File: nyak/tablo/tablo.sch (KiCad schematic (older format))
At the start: 109 parts

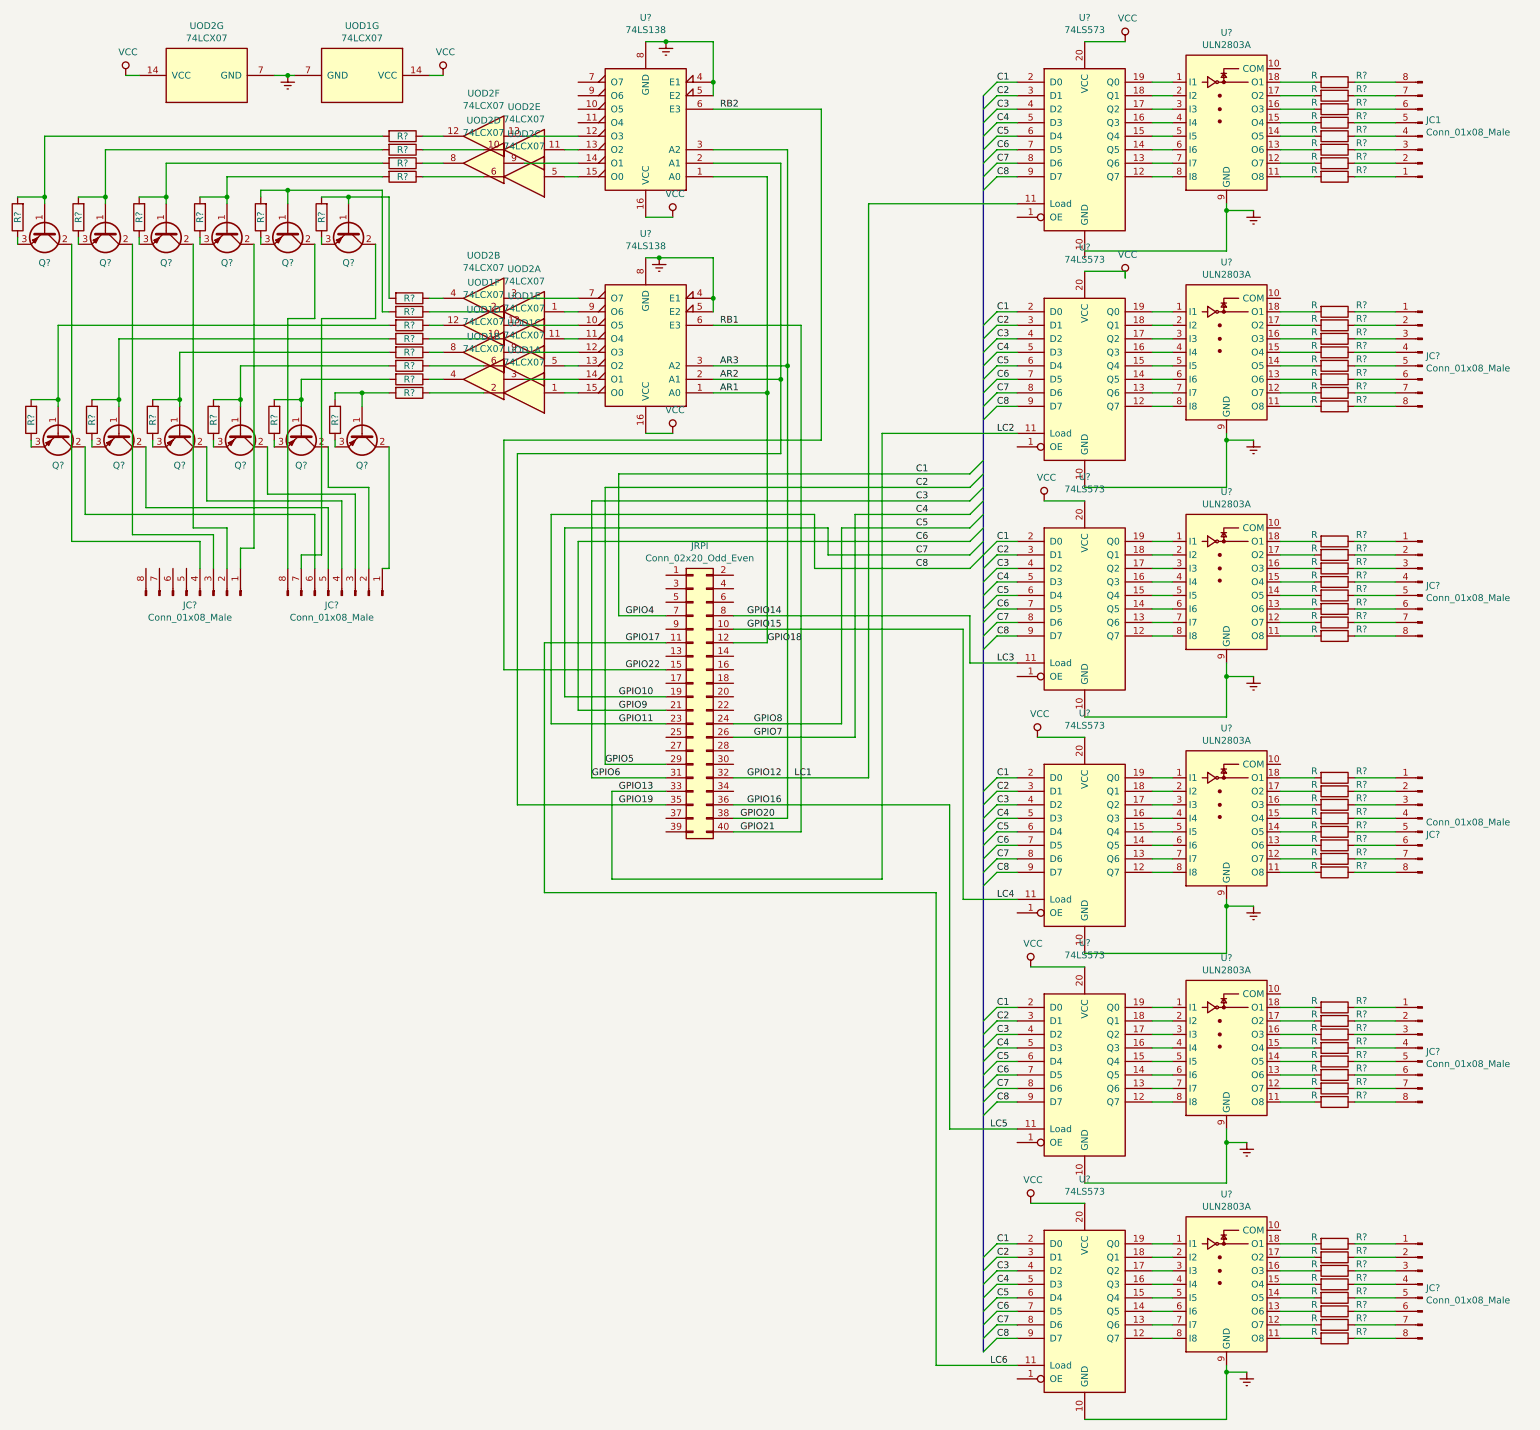
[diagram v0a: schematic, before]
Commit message: footprints added
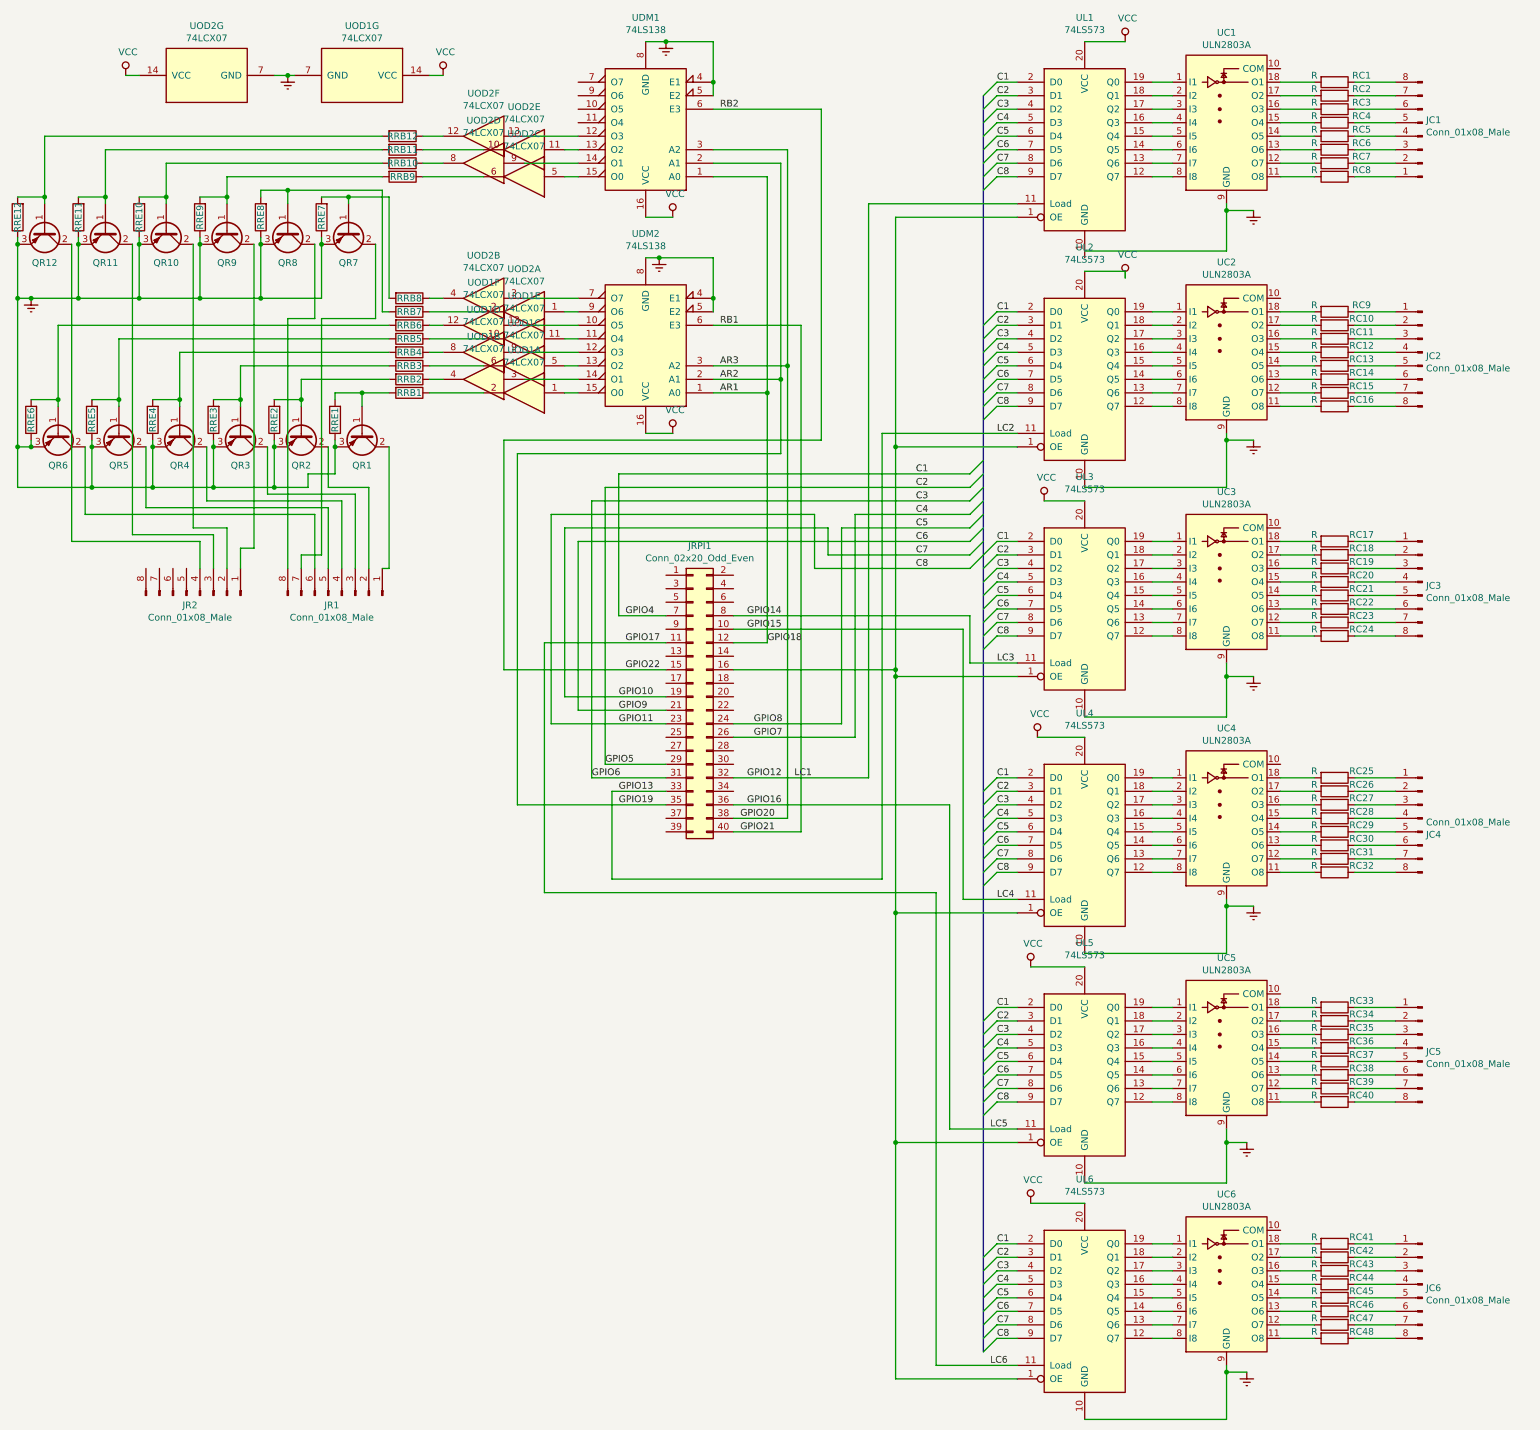
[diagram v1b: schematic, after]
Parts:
- JC1: footprint (none) -> Connector_PinHeader_2.54mm:PinHeader_1x08_P2.54mm_Vertical
- JC2, JC3, JC4, JC5, JC6, JR1, JR2: renamed from JC?; footprint (none) -> Connector_PinHeader_2.54mm:PinHeader_1x08_P2.54mm_Vertical
- JRPI1: renamed from JRPI; footprint (none) -> Connector_PinSocket_2.54mm:PinSocket_2x20_P2.54mm_Vertical
- QR1, QR10, QR11, QR12, QR2, QR3, QR4, QR5, QR6, QR7, QR8, QR9: renamed from Q?; footprint (none) -> Package_TO_SOT_THT:TO-220-3_Vertical
- RC1, RC10, RC11, RC12, RC13, RC14, RC15, RC16, RC17, RC18, RC19, RC2, RC20, RC21, RC22, RC23, RC24, RC25, RC26, RC27, RC28, RC29, RC3, RC30, RC31, RC32, RC33, RC34, RC35, RC36, RC37, RC38, RC39, RC4, RC40, RC41, RC42, RC43, RC44, RC45, RC46, RC47, RC48, RC5, RC6, RC7, RC8, RC9, RRB1, RRB10, RRB11, RRB12, RRB2, RRB3, RRB4, RRB5, RRB6, RRB7, RRB8, RRB9, RRE1, RRE10, RRE11, RRE12, RRE2, RRE3, RRE4, RRE5, RRE6, RRE7, RRE8, RRE9: renamed from R?; footprint (none) -> Resistor_THT:R_Axial_DIN0204_L3.6mm_D1.6mm_P7.62mm_Horizontal
- UC1, UC2, UC3, UC4, UC5, UC6: renamed from U?; footprint (none) -> Package_DIP:DIP-18_W7.62mm
- UDM1, UDM2: renamed from U?; footprint (none) -> Package_DIP:DIP-16_W7.62mm
- UL1, UL2, UL3, UL4, UL5, UL6: renamed from U?; footprint (none) -> Package_DIP:DIP-20_W7.62mm
- UOD1, UOD2: footprint (none) -> Package_DIP:DIP-14_W7.62mm
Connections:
- net Earth: now also QR1.3 (E), QR10.3 (E), QR11.3 (E), QR12.3 (E), QR2.3 (E), QR3.3 (E), QR4.3 (E), QR5.3 (E), QR6.3 (E), QR7.3 (E), QR8.3 (E), QR9.3 (E), RRE1.1, RRE10.1, RRE11.1, RRE12.1, RRE2.1, RRE3.1, RRE4.1, RRE5.1, RRE6.1, RRE7.1, RRE8.1, RRE9.1
- net at UL1.1 (OE): now also JRPI1.16 (Pin_16), UL2.1 (OE), UL3.1 (OE), UL4.1 (OE), UL5.1 (OE), UL6.1 (OE)

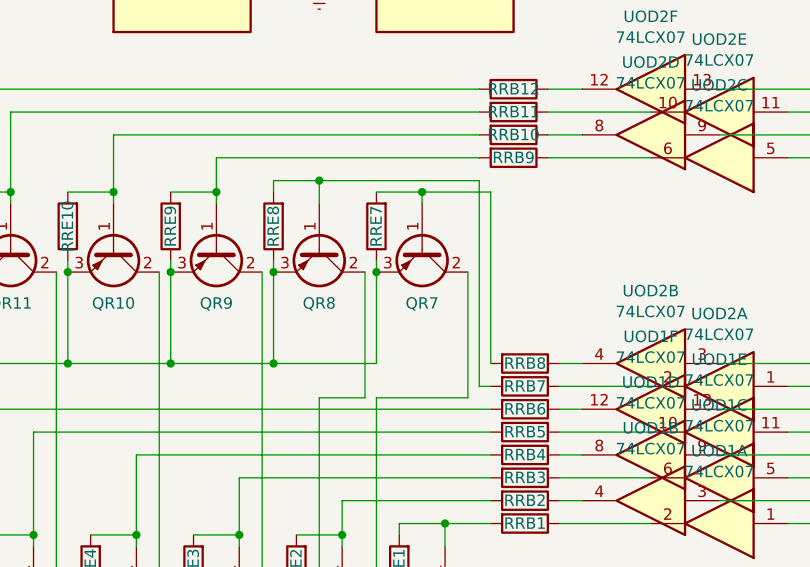
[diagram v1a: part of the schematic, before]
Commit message: more tracks
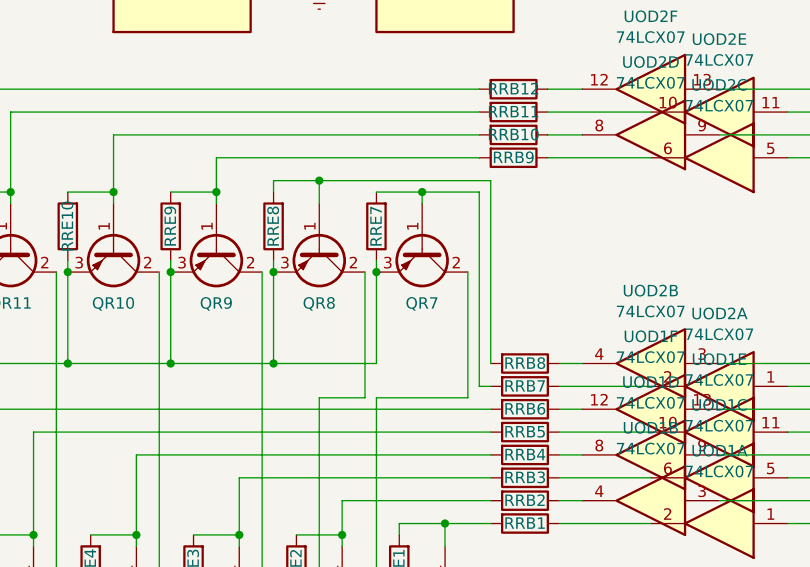
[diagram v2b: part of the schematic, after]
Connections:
- net at QR7.1 (B), RRE7.2: now also RRB7.2; no longer RRB8.2
- net at QR8.1 (B), RRE8.2: now also RRB8.2; no longer RRB7.2
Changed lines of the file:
@@
 	550  2200 550  2150
 Wire Wire Line
-	3300 2600 3300 1850
-Wire Wire Line
-	3300 1850 3000 1850
-Wire Wire Line
 	3000 1850 3000 1900
-Connection ~ 3000 1850
 Wire Wire Line
 	3000 1850 2800 1850
@@
 	3300 2700 3250 2700
 Wire Wire Line
-	3250 2700 3250 1800
-Wire Wire Line
-	3250 1800 2550 1800
-Wire Wire Line
 	2350 1800 2350 1850
 Wire Wire Line
 	2550 1800 2550 1900
-Connection ~ 2550 1800
 Wire Wire Line
 	2550 1800 2350 1800
@@
 Wire Wire Line
 	2900 3900 2900 3700
-Wire Bus Line
-	7700 1100 7700 10400
 Connection ~ 2450 4000
 Connection ~ 2900 3700
@@
 Wire Wire Line
 	650  2600 1000 2600
+Wire Wire Line
+	3300 2600 3300 1800
+Wire Wire Line
+	3300 1800 2550 1800
+Connection ~ 2550 1800
+Wire Wire Line
+	3250 2700 3250 1850
+Wire Wire Line
+	3250 1850 3000 1850
+Wire Bus Line
+	7700 1100 7700 10400
+Connection ~ 3000 1850
 $EndSCHEMATC

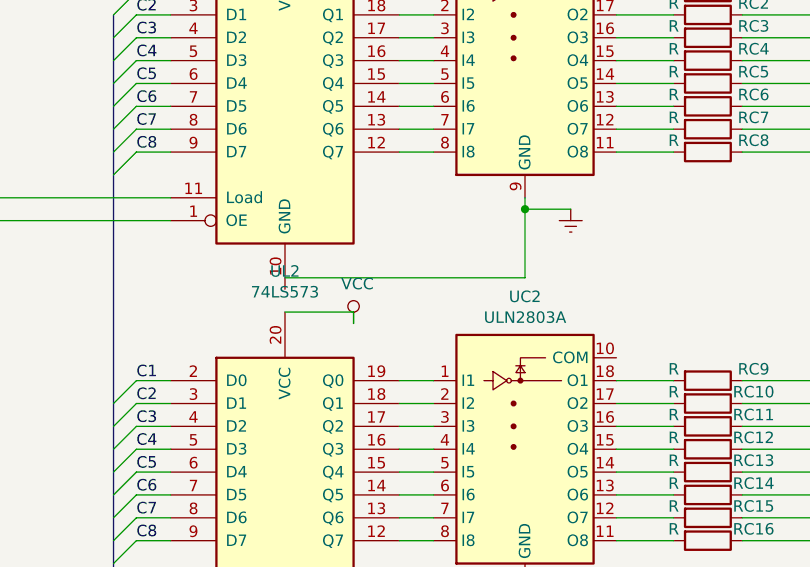
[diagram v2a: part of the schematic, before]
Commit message: more pcb
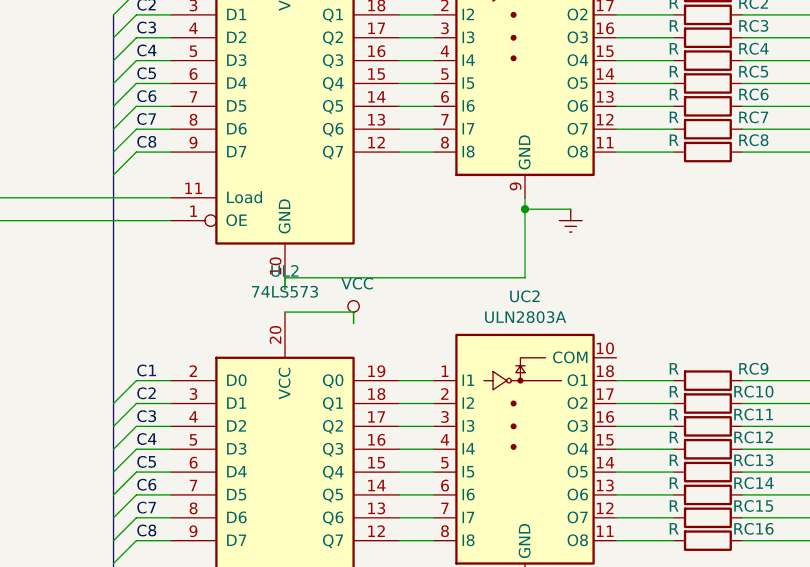
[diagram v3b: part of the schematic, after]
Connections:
- net Earth: now also UL1.10 (GND)
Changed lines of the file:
@@
 EESchema Schematic File Version 4
-LIBS:tablo-cache
-EELAYER 26 0
+EELAYER 30 0
 EELAYER END
 $Descr A3 16535 11693
@@
 	8950 10300 9100 10300
 Wire Wire Line
-	8450 2250 9500 2250
-Wire Wire Line
 	9500 2250 9500 1950
-Wire Wire Line
-	8450 4000 9500 4000
-Wire Wire Line
-	9500 4000 9500 3650
 Wire Wire Line
 	8450 5700 9500 5700
@@
 Wire Wire Line
 	9700 3650 9500 3650
-Connection ~ 9500 3650
 Wire Wire Line
 	9500 3650 9500 3600
@@
 Wire Wire Line
 	3250 1850 3000 1850
+Connection ~ 3000 1850
+Connection ~ 9500 3650
+Wire Wire Line
+	9500 4000 9500 3650
+Wire Wire Line
+	8450 4000 9500 4000
+Wire Wire Line
+	9500 2250 8450 2250
+Wire Wire Line
+	8450 2250 8450 2300
 Wire Bus Line
 	7700 1100 7700 10400
-Connection ~ 3000 1850
 $EndSCHEMATC
